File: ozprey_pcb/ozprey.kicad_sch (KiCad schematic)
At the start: 4 parts, among them SW43 SK12D07VG4, U1 nice_nano

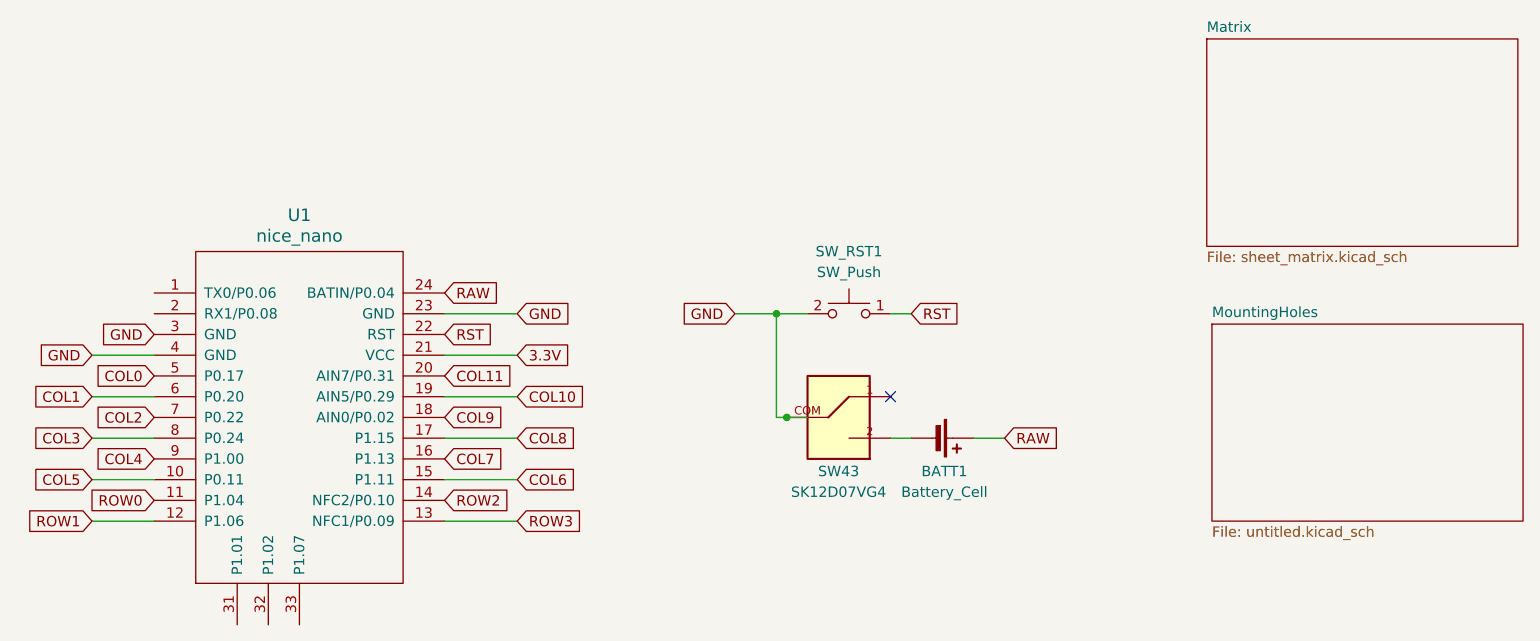
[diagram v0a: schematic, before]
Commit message: major changes, add plate
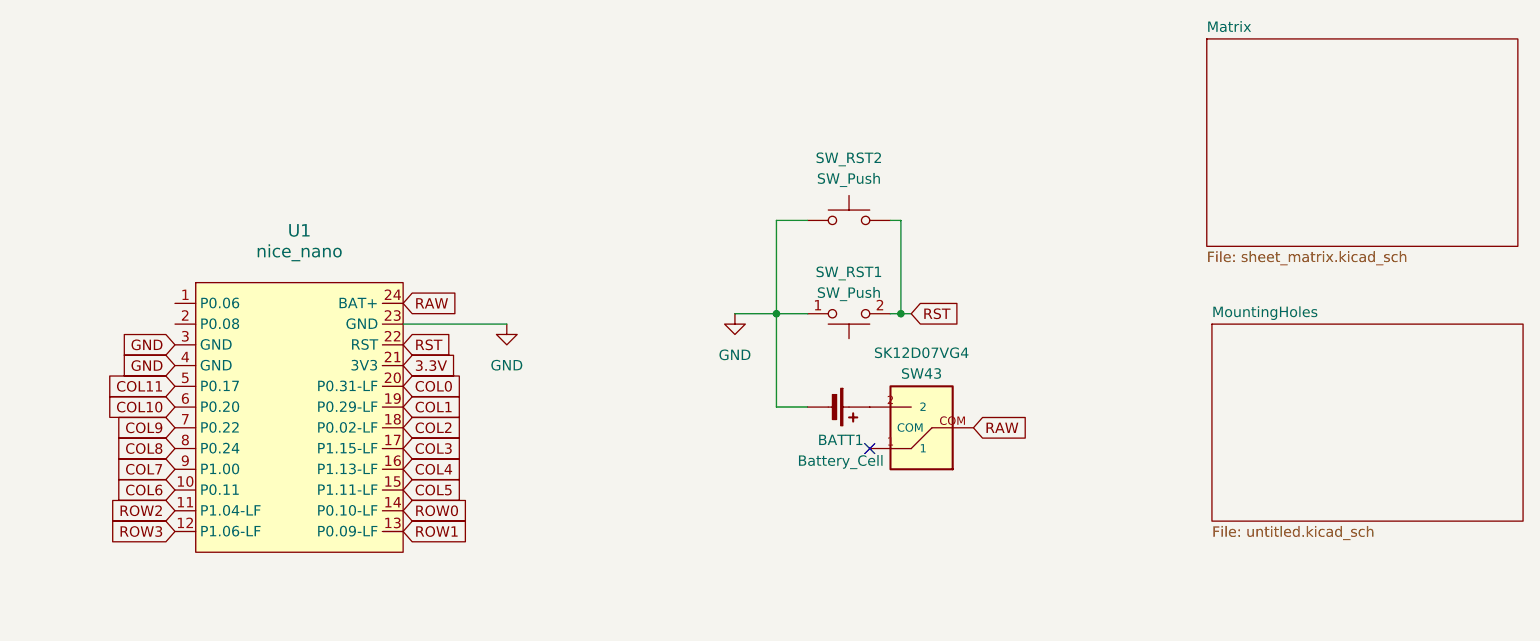
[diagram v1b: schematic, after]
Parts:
- added SW_RST2: SW_Push, itsdmd:SW-T_SPST_TL3342, symbol Switch:SW_Push
- BATT1: footprint Keyboard:Battery_pads -> itsdmd:Battery_Pads-dual-side
- SW43: footprint Switch:SK12D07VG4 -> itsdmd:SW-S_SK12D07VG4; symbol SK12D07VG4:SK12D07VG4 -> itsdmd:SK12D07VG4
- SW_RST1: footprint Switch:KG1 -> itsdmd:SW-S_7.4x2.6-4pad-smd
- U1: footprint ProMicro:nice_nano -> itsdmd:MCB_nice-nano_flip; symbol nice_nano:nice_nano -> itsdmd:nice_nano; now left out of the parts list
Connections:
- net COL0: now also U1.20 (P0.31-LF); no longer U1.5 (P0.17)
- net COL1: now also U1.19 (P0.29-LF); no longer U1.6 (P0.20)
- net COL10: now also U1.6 (P0.20); no longer U1.19 (AIN5/P0.29)
- net COL11: now also U1.5 (P0.17); no longer U1.20 (AIN7/P0.31)
- net COL2: now also U1.18 (P0.02-LF); no longer U1.7 (P0.22)
- net COL3: now also U1.17 (P1.15-LF); no longer U1.8 (P0.24)
- net COL4: now also U1.16 (P1.13-LF); no longer U1.9 (P1.00)
- net COL5: now also U1.15 (P1.11-LF); no longer U1.10 (P0.11)
- net COL6: now also U1.10 (P0.11); no longer U1.15 (P1.11)
- net COL7: now also U1.9 (P1.00); no longer U1.16 (P1.13)
- net COL8: now also U1.8 (P0.24); no longer U1.17 (P1.15)
- net COL9: now also U1.7 (P0.22); no longer U1.18 (AIN0/P0.02)
- net GND: now also BATT1.2 (-), SW_RST1.1, SW_RST2.1; no longer SW43.COM, SW_RST1.2
- net RAW: now also SW43.COM; no longer BATT1.1 (+)
- net ROW0: now also U1.14 (P0.10-LF); no longer U1.11 (P1.04)
- net ROW1: now also U1.13 (P0.09-LF); no longer U1.12 (P1.06)
- net ROW2: now also U1.11 (P1.04-LF); no longer U1.14 (NFC2/P0.10)
- net ROW3: now also U1.12 (P1.06-LF); no longer U1.13 (NFC1/P0.09)
- net RST: now also SW_RST1.2, SW_RST2.2; no longer SW_RST1.1
- net at SW43.2: now also BATT1.1 (+); no longer BATT1.2 (-)
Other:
- moved on the sheet: BATT1, SW_RST1
